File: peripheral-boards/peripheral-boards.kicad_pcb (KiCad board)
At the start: 4 copper layers, 50.8 x 45.7 mm, 59 parts, among them J8 FTSH-107-01-F-DV-K-P-TR, SW1 Y97KT23B5NAFP, SW5 A6H-4101, U12 INA826AIDR, U13 REF35160QDBVR, U14 TCA9406DC, U2 TCA9406DC, U3 STM32G441KBTx, U4 ISO1044DUB, U5 MCP1703AT-5002E/CB, U6 MCP1703AT-3302E/CB, U8 LMV331, Y1 ECS-240-8-37B-CKY-TR

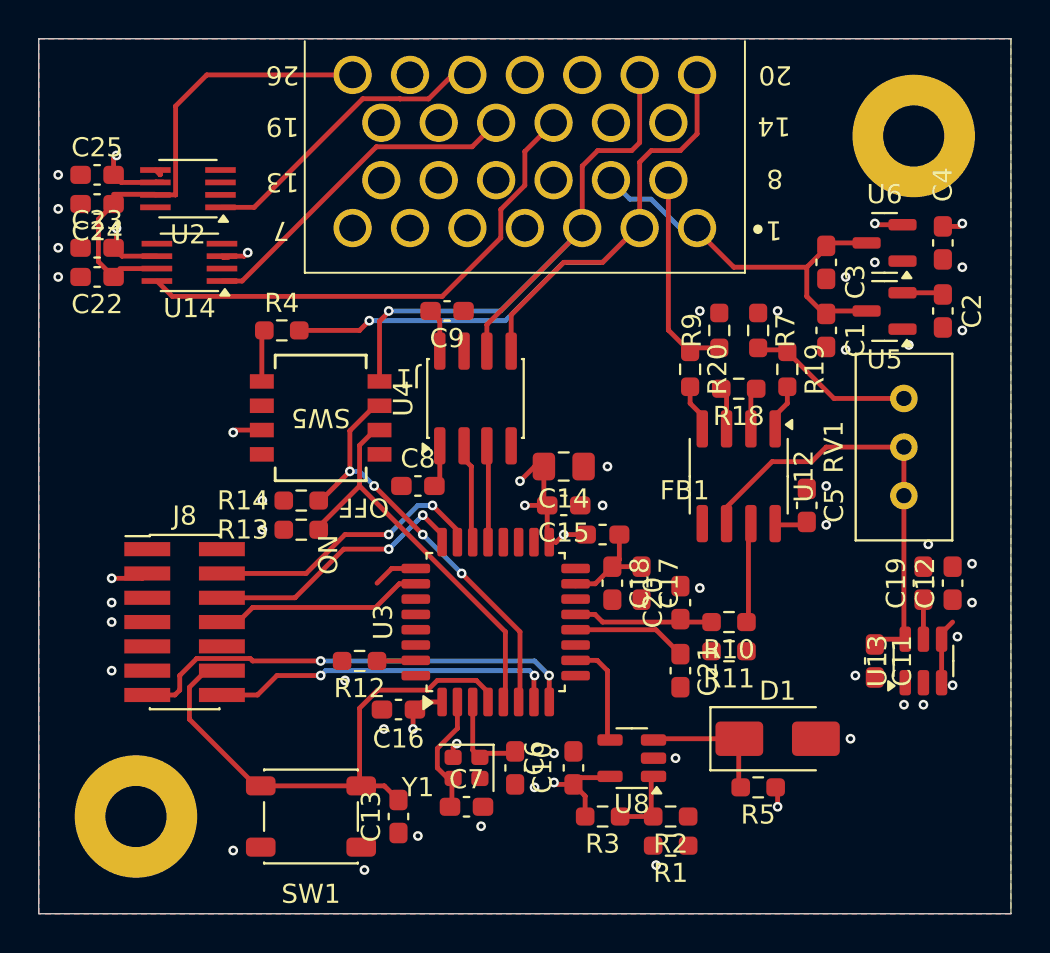
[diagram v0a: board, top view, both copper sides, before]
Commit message: Prepared peripheral board for order
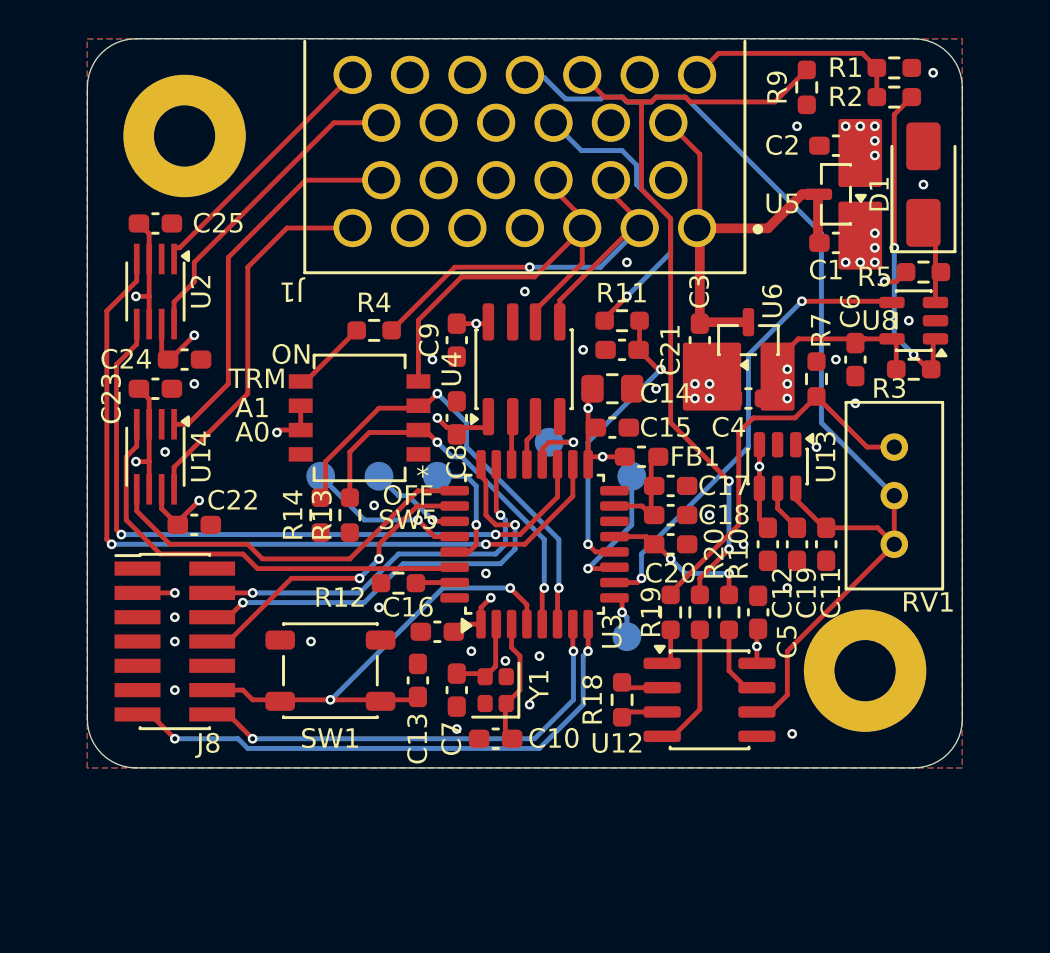
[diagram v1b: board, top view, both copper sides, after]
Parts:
- added G***: , FS_4_Global_Footprint_Library:FORMULA SLUG TITLE, B.Cu at (139.7, 132.1)
- added TP1: PA4, TestPoint:TestPoint_Pad_D1.5mm, B.Cu at (150.1, 130.3)
- added TP2: PA6, TestPoint:TestPoint_Pad_D1.5mm, B.Cu at (150.4, 121.9)
- added TP3: PA10, TestPoint:TestPoint_Pad_D1.5mm, B.Cu at (146.1, 120.1)
- added TP4: PB4, TestPoint:TestPoint_Pad_D1.5mm, B.Cu at (137.2, 121.9)
- added TP5: PB6, TestPoint:TestPoint_Pad_D1.5mm, B.Cu at (140.2, 121.9)
- added TP6: PB7, TestPoint:TestPoint_Pad_D1.5mm, B.Cu at (134.1, 121.9)
- R19, R20: value 16K -> 10k
- SW5: footprint Library:SW_A6H-4101_OMR -> FS_4_Global_Footprint_Library:SW_A6H-4101_OMR
- moved R1 42.3 mm to (164.1, 100.6), turned to 0 degrees
- moved R2 39.4 mm to (164.1, 102.1), turned to 0 degrees
- moved H2 35.7 mm to (127.0, 104.1)
- moved D1 29.9 mm to (165.6, 106.7), turned to 90 degrees
- moved R3 28.5 mm to (165.1, 116.3)
- moved R5 28.3 mm to (165.6, 111.3), turned to 0 degrees
- moved H1 28.1 mm to (162.6, 132.1)
- moved U8 27.2 mm to (165.1, 113.8)
- moved C6 25.9 mm to (162.1, 115.8), turned to -90 degrees
- moved R11 18.2 mm to (149.9, 113.8), turned to 0 degrees
- moved R18 17.4 mm to (149.9, 133.6), turned to -90 degrees
- moved C21 17.0 mm to (149.9, 115.3), turned to 180 degrees
- moved R19 14.1 mm to (152.4, 129.0)
- moved C22 13.9 mm to (127.5, 124.5), turned to 0 degrees
- moved R9 13.5 mm to (159.5, 101.6), turned to -90 degrees
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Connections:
- J1 pad 10: /Wheel_Speed_Out -> CANH
- J1 pad 11: GND -> +5V
- J1 pad 12: +3V3 -> GND
- J1 pad 13: Net-(J1D-1) -> Net-(U14-SDA_B)
- J1 pad 14: GND -> +12V
- J1 pad 15: GND -> +3V3
- J1 pad 16: Net-(U14-SCL_B) -> Net-(J1-Pad16)
- J1 pad 17: Net-(U14-SDA_B) -> GND
- J1 pad 18: +5V -> GND
- J1 pad 19: +5V -> Net-(U2-SCL_B)
- J1 pad 20: CANH -> /Wheel_Speed_Out
- J1 pad 21: CANL -> GND
- J1 pad 22: GND -> /Vin+
- J1 pad 23: GND -> /1V6_Vref
- J1 pad 24: Net-(U2-SDA_B) -> unconnected-(J1-Pad24)
- J1 pad 25: Net-(U2-SCL_B) -> +5V
- J1 pad 26: +5V -> Net-(U2-SDA_B)
- J1 pad 6: unconnected-(J1-Pad6) -> +5V
- J1 pad 7: /1V6_Vref -> Net-(U14-SCL_B)
- J1 pad 8: /Vin+ -> GND
- J1 pad 9: +12V -> CANL
- R11 pad 1: Net-(J1D-1) -> Net-(J1-Pad16)
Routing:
- net 1x8_TireTemp_Sensor_SDA: track 0.00 -> 42.5 mm, vias 0 -> 2
- net 1x8_TireTemp_Sensor_SCL: track 0.60 -> 36.9 mm, vias 0 -> 2
- net /1V6_Vref: track 23.2 -> 54.6 mm
- net /Vin+: track 11.1 -> 41.5 mm, vias 0 -> 2
- net +3V3: track 40.3 -> 64.3 mm, vias 17 -> 14
- net 1x1_TireTemp_Sensor_SDA: track 0.00 -> 23.4 mm
- net +5V: track 29.1 -> 8.66 mm, vias 0 -> 8
- net wheel speed: track 5.57 -> 24.0 mm, vias 0 -> 2
- net CANL: track 41.4 -> 23.8 mm
- net 1x1_TireTemp_Sensor_SCL: track 2.34 -> 19.9 mm
- net Net-(U2-SCL_B): track 0.00 -> 16.5 mm
- net Net-(J1-Pad16): track 0.00 -> 15.5 mm, vias 0 -> 1
- net CANH: track 35.5 -> 21.2 mm, vias 1 -> 0
- net Net-(U8-+): track 3.92 -> 16.7 mm, vias 0 -> 2
- net /Wheel_Speed_Out: track 0.00 -> 11.7 mm
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- added copper zone on In2.Cu, net +5V
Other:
- board size 50.8 x 45.7 mm -> 45.7 x 38.1 mm
- board text added: "*"
- board text added: "A0"
- board text added: "A1"
- board text added: "TRM"
